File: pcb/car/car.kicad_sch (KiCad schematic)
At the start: 9 parts

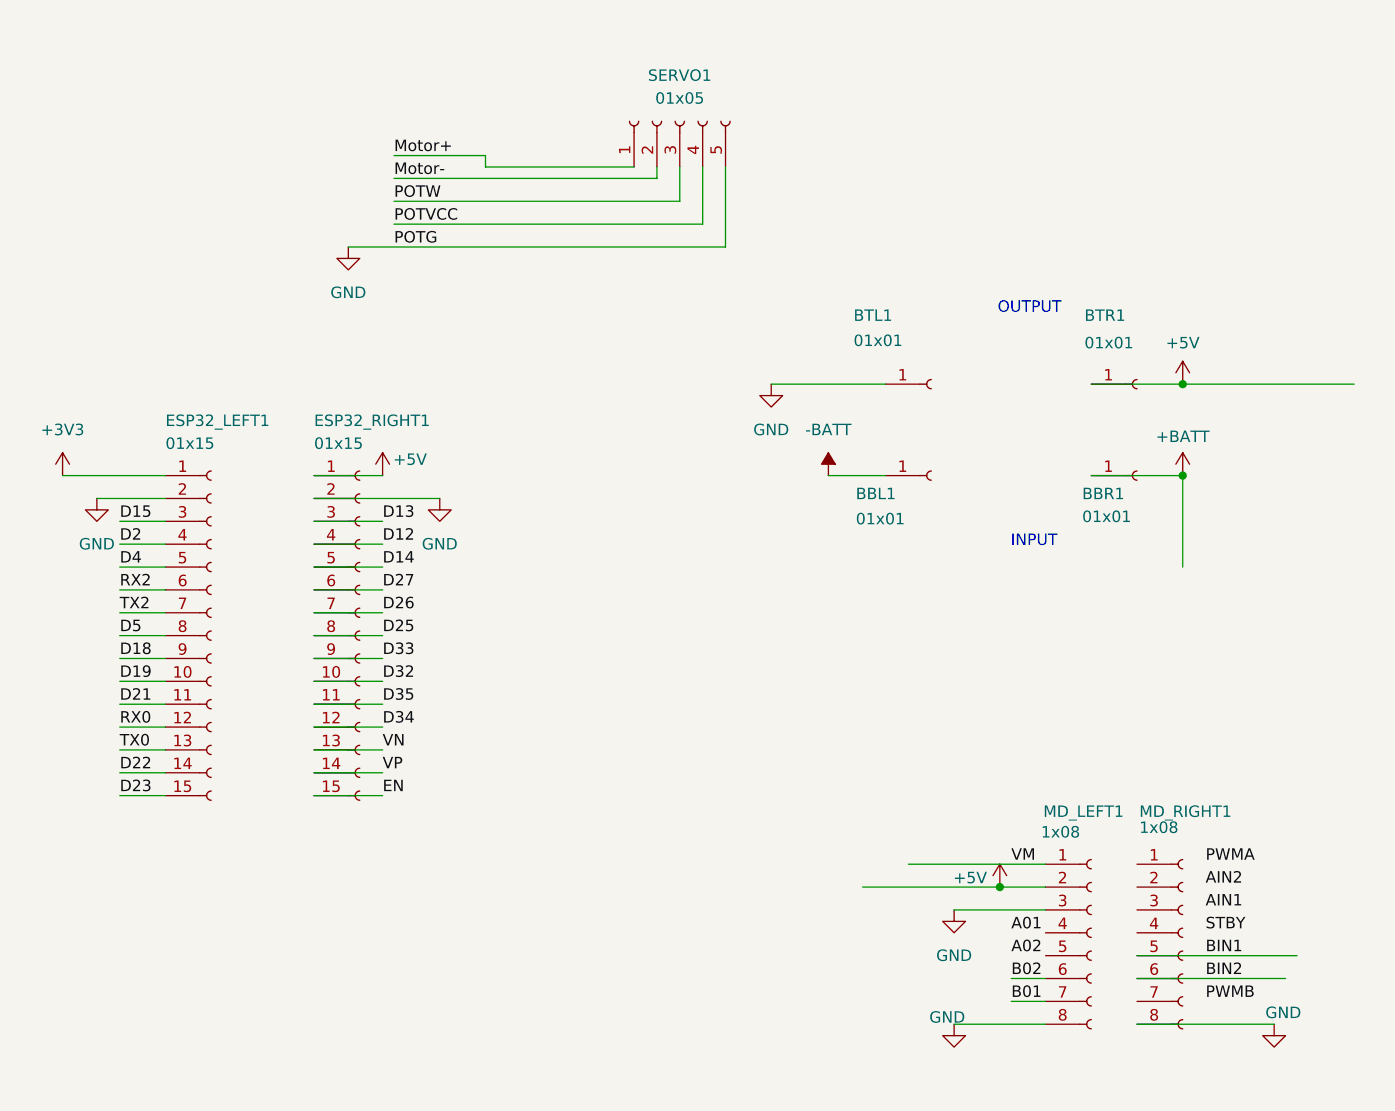
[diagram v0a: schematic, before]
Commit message: feat: cleaning up pdb
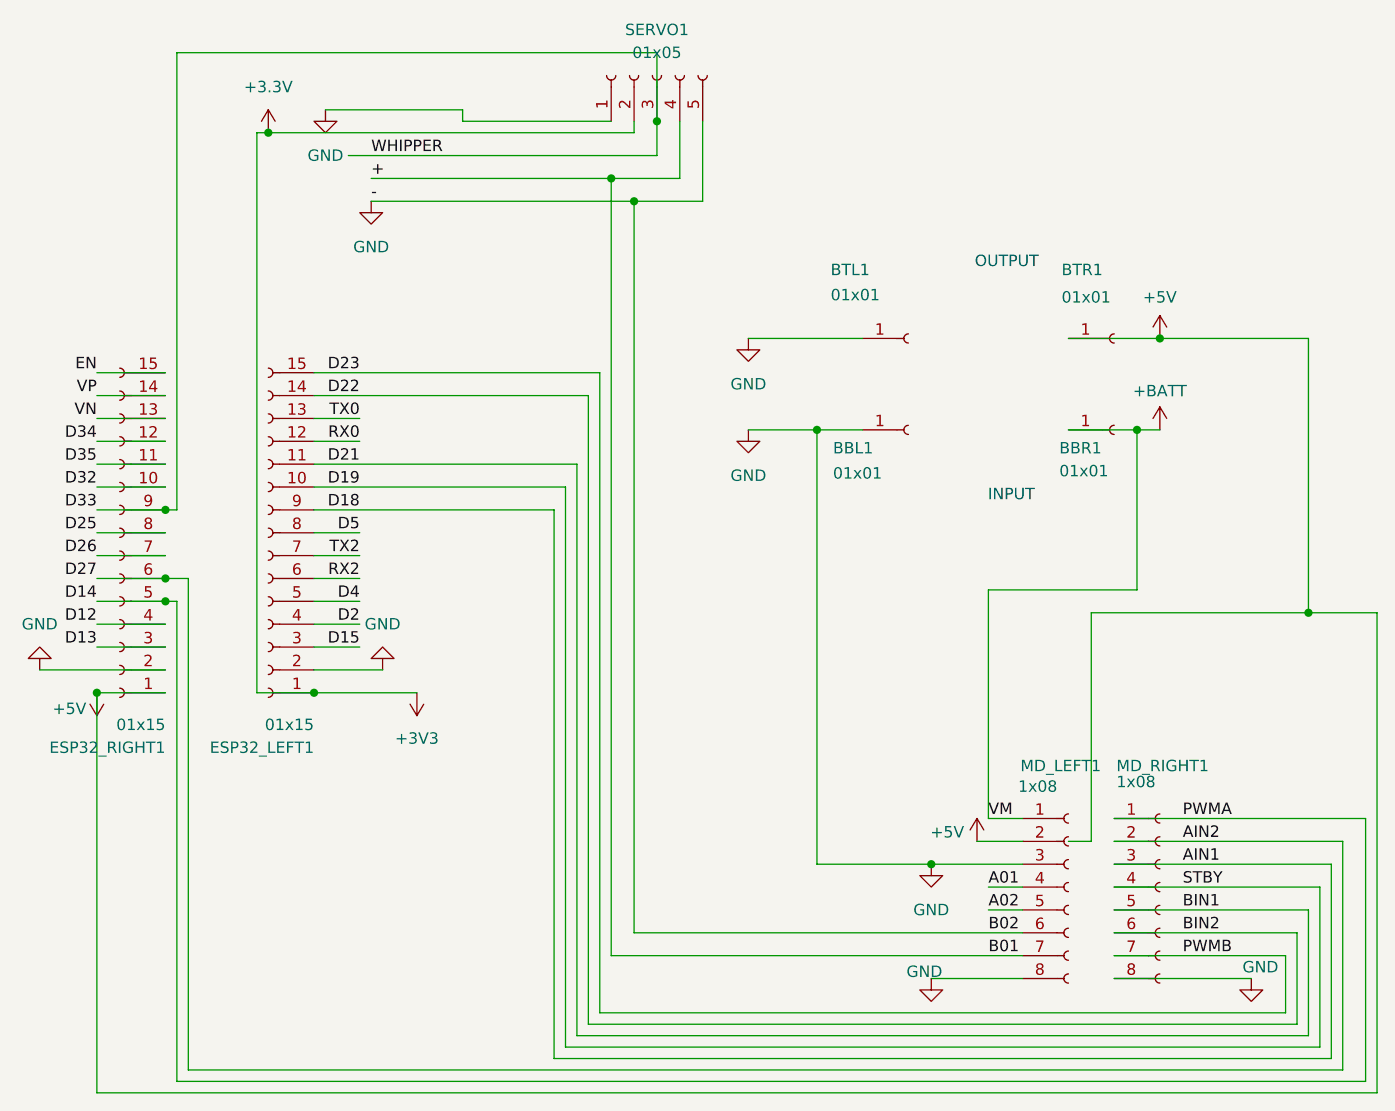
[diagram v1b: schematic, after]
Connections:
- net -BATT is gone; now on net GND: BBL1.1 (Pin_1)
- net B02 is gone; now on net GND: MD_LEFT1.6 (Pin_6)
- net D18 is gone; now on net AIN1: ESP32_LEFT1.9 (Pin_9)
- net D21 is gone; now on net BIN1: ESP32_LEFT1.11 (Pin_11)
- net D22 is gone; now on net BIN2: ESP32_LEFT1.14 (Pin_14)
- net D27 is gone; now on net AIN2: ESP32_RIGHT1.6 (Pin_6)
- net Motor+ is gone; now on net GND: SERVO1.1 (Pin_1)
- net Motor- is gone; now on net +3.3V: SERVO1.2 (Pin_2)
- net POTVCC is gone; now on net +: SERVO1.4 (Pin_4)
- net POTW is gone; now on net D33: SERVO1.3 (Pin_3)
- net VM is gone; now on net +BATT: MD_LEFT1.1 (Pin_1)
- net A01: now also MD_LEFT1.4 (Pin_4)
- net A02: now also MD_LEFT1.5 (Pin_5)
- net AIN1: now also MD_RIGHT1.3 (Pin_3)
- net AIN2: now also MD_RIGHT1.2 (Pin_2)
- net D14: now also MD_RIGHT1.1 (Pin_1)
- net D19: now also MD_RIGHT1.4 (Pin_4)
- net D23: now also MD_RIGHT1.7 (Pin_7)
- net +3V3 renamed +3.3V
- net B01 renamed +
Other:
- moved on the sheet: BBL1, BBR1, BTL1, BTR1, ESP32_LEFT1, ESP32_RIGHT1, MD_LEFT1, MD_RIGHT1, SERVO1
